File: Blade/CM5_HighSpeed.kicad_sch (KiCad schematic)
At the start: 2 parts, among them J7 Conn_01x22_Female

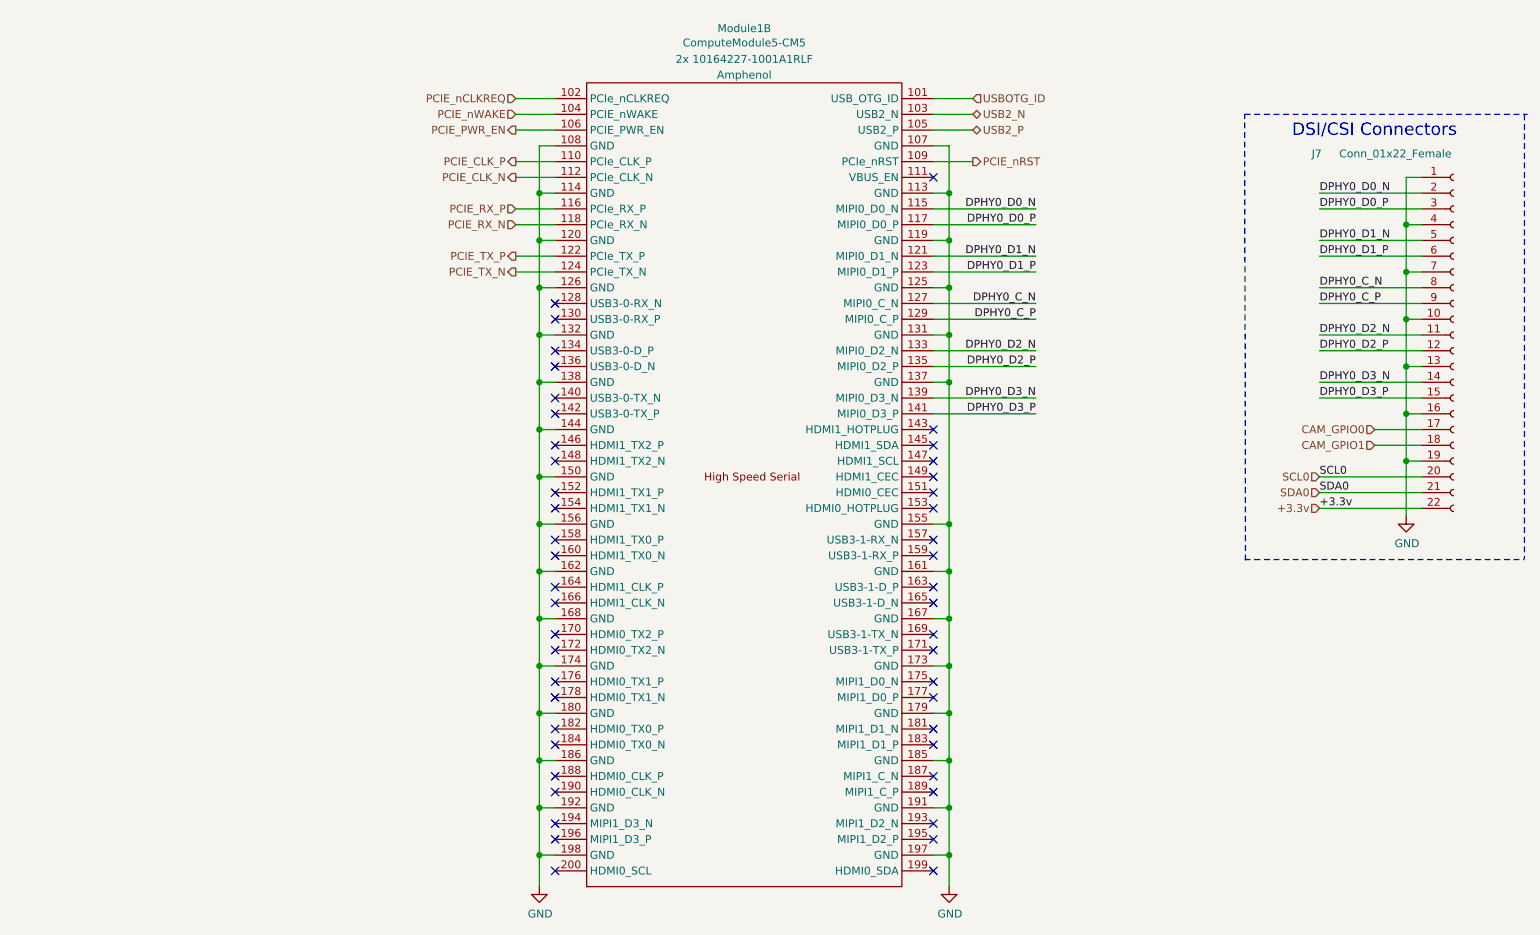
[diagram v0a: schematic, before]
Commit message: Fixing Blade Carrier Board
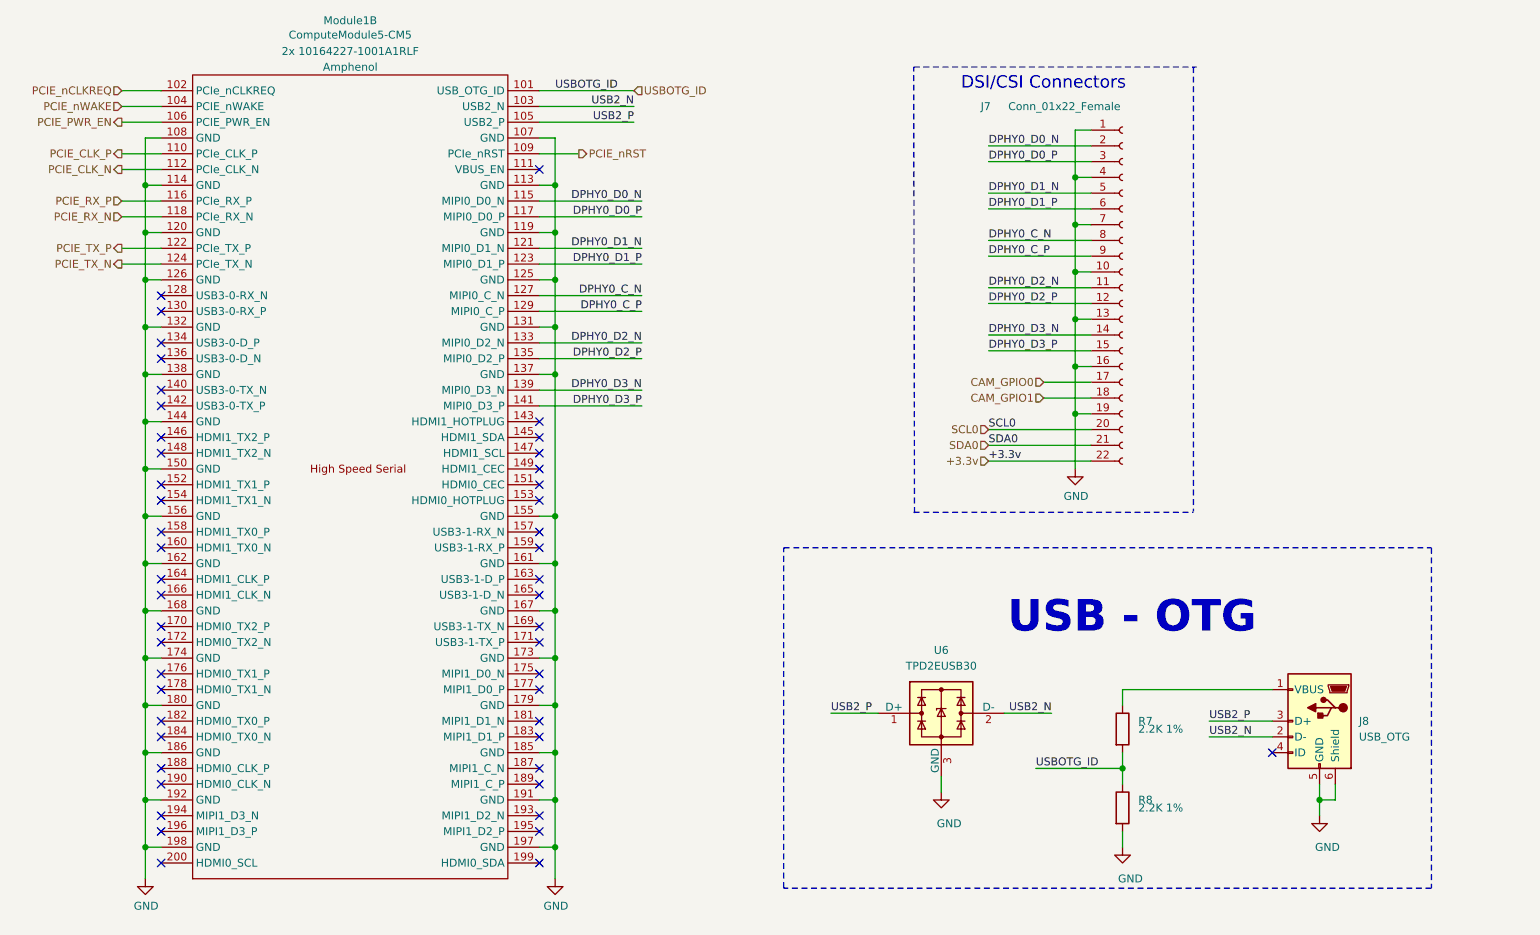
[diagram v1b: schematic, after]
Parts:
- added J8: USB_OTG, CM4IO:USB_Micro-B_EDAC_UCON00686, symbol Connector:USB_OTG
- added R7, R8: 2.2K 1%, Resistor_SMD:R_0603_1608Metric_Pad0.98x0.95mm_HandSolder, symbol Device:R
- added U6: TPD2EUSB30, Package_TO_SOT_SMD:Texas_DRT-3, symbol Power_Protection:TPD2EUSB30
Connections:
- net GND: now also J8.5 (GND), J8.6 (Shield), R8.2, U6.3 (GND)
- net USB2_N: now also J8.2 (D-), U6.2 (D-)
- net USB2_P: now also J8.3 (D+), U6.1 (D+)
- net USBOTG_ID: now also R7.2, R8.1
- new net: J8.1 (VBUS), R7.1
- no-connect marks 47 -> 48
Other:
- note added: "USB - OTG"
- moved on the sheet: J7, Module1B
